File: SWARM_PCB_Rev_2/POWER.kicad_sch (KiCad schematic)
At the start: 70 parts

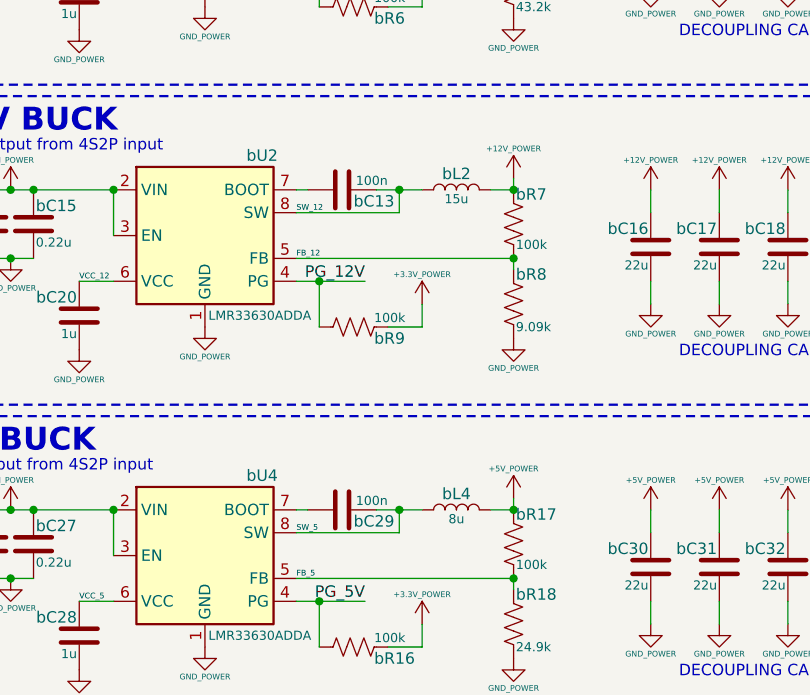
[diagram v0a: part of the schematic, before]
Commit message: Revert "to delete"
This reverts commit 543c70bcba01ecf78262208d4f10808184dfb0ad.
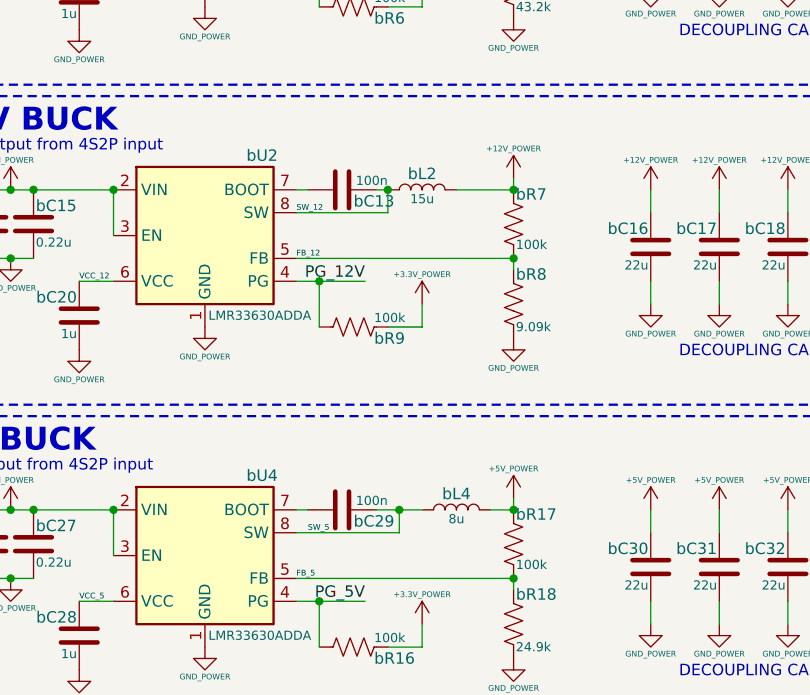
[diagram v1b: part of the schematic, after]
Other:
- moved on the sheet: bL2
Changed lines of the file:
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@@
 	)
 	(junction
-		(at 63.5 58.42)
-		(diameter 0)
-		(color 0 0 0 0)
-	)
-	(junction
-		(at 76.2 58.42)
+		(at 62.23 58.42)
 		(diameter 0)
 		(color 0 0 0 0)
@@
 	)
 	(junction
+		(at 76.2 58.42)
+		(diameter 0)
+		(color 0 0 0 0)
+	)
+	(junction
 		(at 20.32 58.42)
 		(diameter 0)
@@
 	(wire
 		(pts
-			(xy 52.07 60.96) (xy 63.5 60.96)
+			(xy 52.07 60.96) (xy 62.23 60.96)
 		)
 		(stroke
@@
 	(wire
 		(pts
-			(xy 73.66 58.42) (xy 76.2 58.42)
+			(xy 69.85 58.42) (xy 76.2 58.42)
 		)
 		(stroke
@@
 	(wire
 		(pts
-			(xy 66.04 58.42) (xy 63.5 58.42)
-		)
-		(stroke
-			(width 0)
-			(type default)
-		)
-	)
-	(wire
-		(pts
 			(xy 20.32 58.42) (xy 22.86 58.42)
 		)
@@
 	(wire
 		(pts
-			(xy 63.5 60.96) (xy 63.5 58.42)
+			(xy 62.23 60.96) (xy 62.23 58.42)
 		)
 		(stroke
@@
 	(wire
 		(pts
-			(xy 60.96 58.42) (xy 63.5 58.42)
+			(xy 62.23 58.42) (xy 60.96 58.42)
 		)
 		(stroke
@@
 	)
 	(label "SW_5"
-		(at 52.07 96.52 0)
+		(at 53.34 96.52 0)
 		(effects
 			(font
@@
 	(symbol
 		(lib_id "Device:L")
-		(at 69.85 58.42 90)
+		(at 66.04 58.42 90)
 		(unit 1)
 		(body_style 1)
@@
 		(dnp no)
 		(property "Reference" "bL2"
-			(at 69.85 56.642 90)
+			(at 66.04 56.642 90)
 			(show_name no)
 			(do_not_autoplace no)
@@
 		)
 		(property "Value" "15u"
-			(at 69.85 59.436 90)
+			(at 66.04 59.436 90)
 			(show_name no)
 			(do_not_autoplace no)
@@
 		)
 		(property "Footprint" "Inductor_SMD:L_Wuerth_MAPI-5030"
-			(at 69.85 58.42 0)
+			(at 66.04 58.42 0)
 			(hide yes)
 			(show_name no)
@@
 		)
 		(property "Datasheet" ""
-			(at 69.85 58.42 0)
+			(at 66.04 58.42 0)
 			(hide yes)
 			(show_name no)
@@
 		)
 		(property "Description" "Inductor"
-			(at 69.85 58.42 0)
+			(at 66.04 58.42 0)
 			(hide yes)
 			(show_name no)
@@
 		)
 		(property "Manufacturer" "Würth Elektronik"
-			(at 3.81 0 0)
+			(at 0 0 0)
 			(hide yes)
 			(show_name no)
@@
 		)
 		(property "MPN" "7447799150"
-			(at 3.81 0 0)
+			(at 0 0 0)
 			(hide yes)
 			(show_name no)
